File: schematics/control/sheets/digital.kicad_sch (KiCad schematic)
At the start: 22 parts, among them U1 Pico, U3 TL072, U4 CD4051B, U5 MCP4822

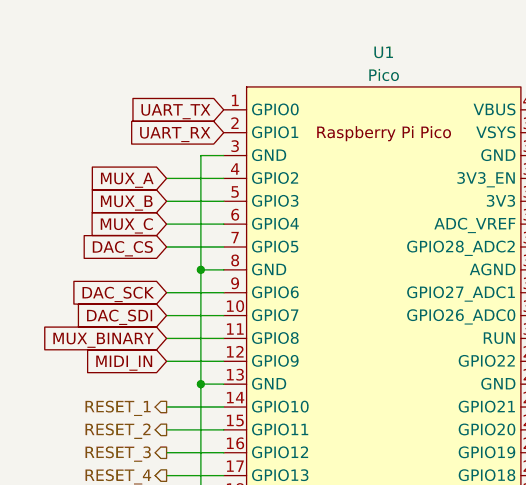
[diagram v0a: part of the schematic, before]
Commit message: Updated schem. + added JLCPCB gerbers
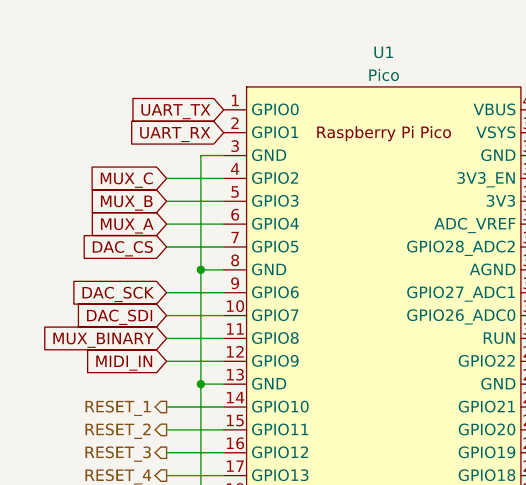
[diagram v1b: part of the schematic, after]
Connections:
- net MUX_A: now also U1.6 (GPIO4); no longer U1.4 (GPIO2)
- net MUX_C: now also U1.4 (GPIO2); no longer U1.6 (GPIO4)
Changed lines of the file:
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@@
     )
   )
-  (global_label "MUX_A" (shape input) (at 31.75 39.37 180) (fields_autoplaced)
+  (global_label "MUX_A" (shape input) (at 31.75 44.45 180) (fields_autoplaced)
     (effects (font (size 1.27 1.27)) (justify right))
-    (property "Intersheetrefs" "${INTERSHEET_REFS}" (at 23.2893 39.2906 0)
+    (property "Intersheetrefs" "${INTERSHEET_REFS}" (at 23.2893 44.3706 0)
       (effects (font (size 1.27 1.27)) (justify right) hide)
     )
   )
-  (global_label "MUX_C" (shape input) (at 31.75 44.45 180) (fields_autoplaced)
+  (global_label "MUX_C" (shape input) (at 31.75 39.37 180) (fields_autoplaced)
     (effects (font (size 1.27 1.27)) (justify right))
-    (property "Intersheetrefs" "${INTERSHEET_REFS}" (at 23.1079 44.3706 0)
+    (property "Intersheetrefs" "${INTERSHEET_REFS}" (at 23.1079 39.2906 0)
       (effects (font (size 1.27 1.27)) (justify right) hide)
     )
